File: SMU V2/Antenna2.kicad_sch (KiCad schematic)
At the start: 9 parts, among them J1101 SMA

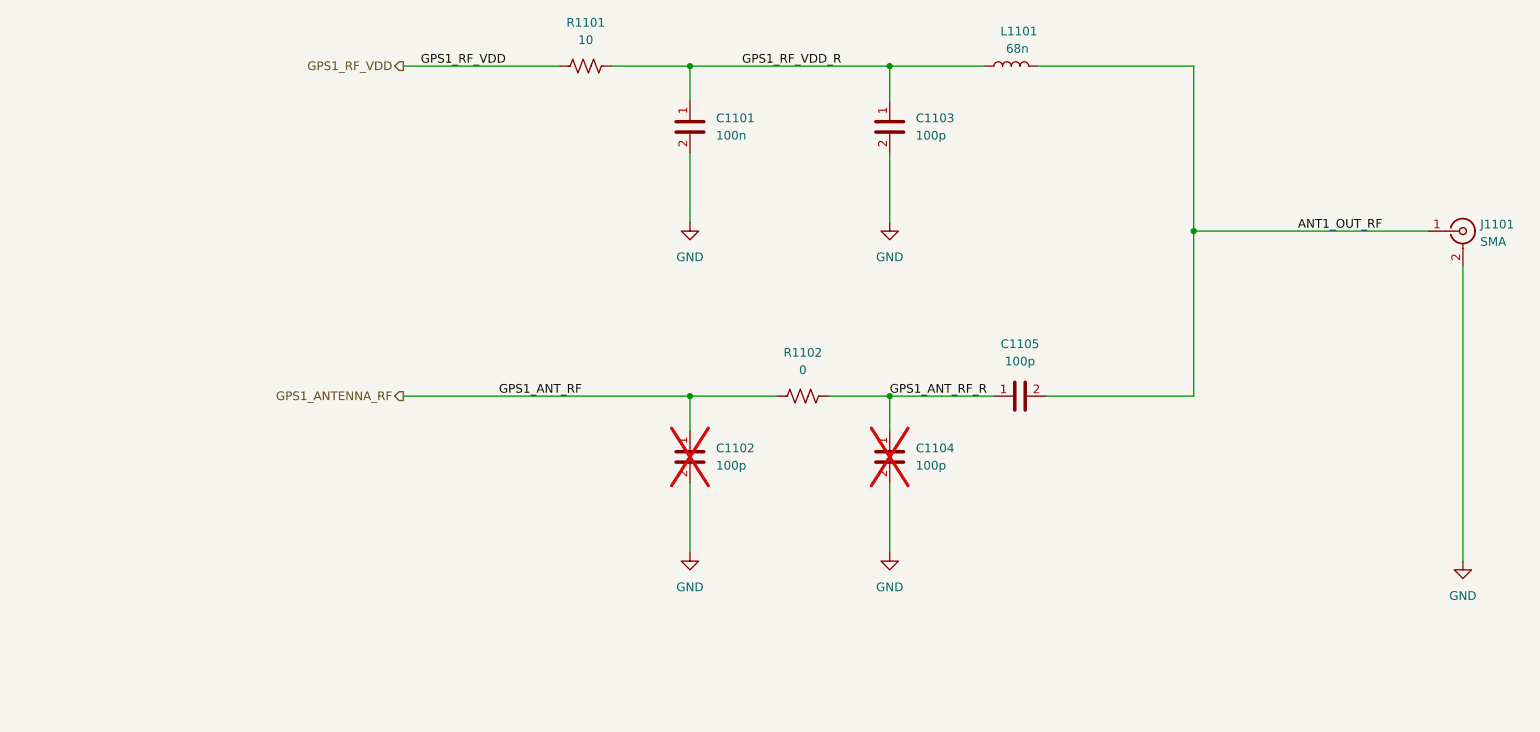
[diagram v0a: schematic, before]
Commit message: v2 layout
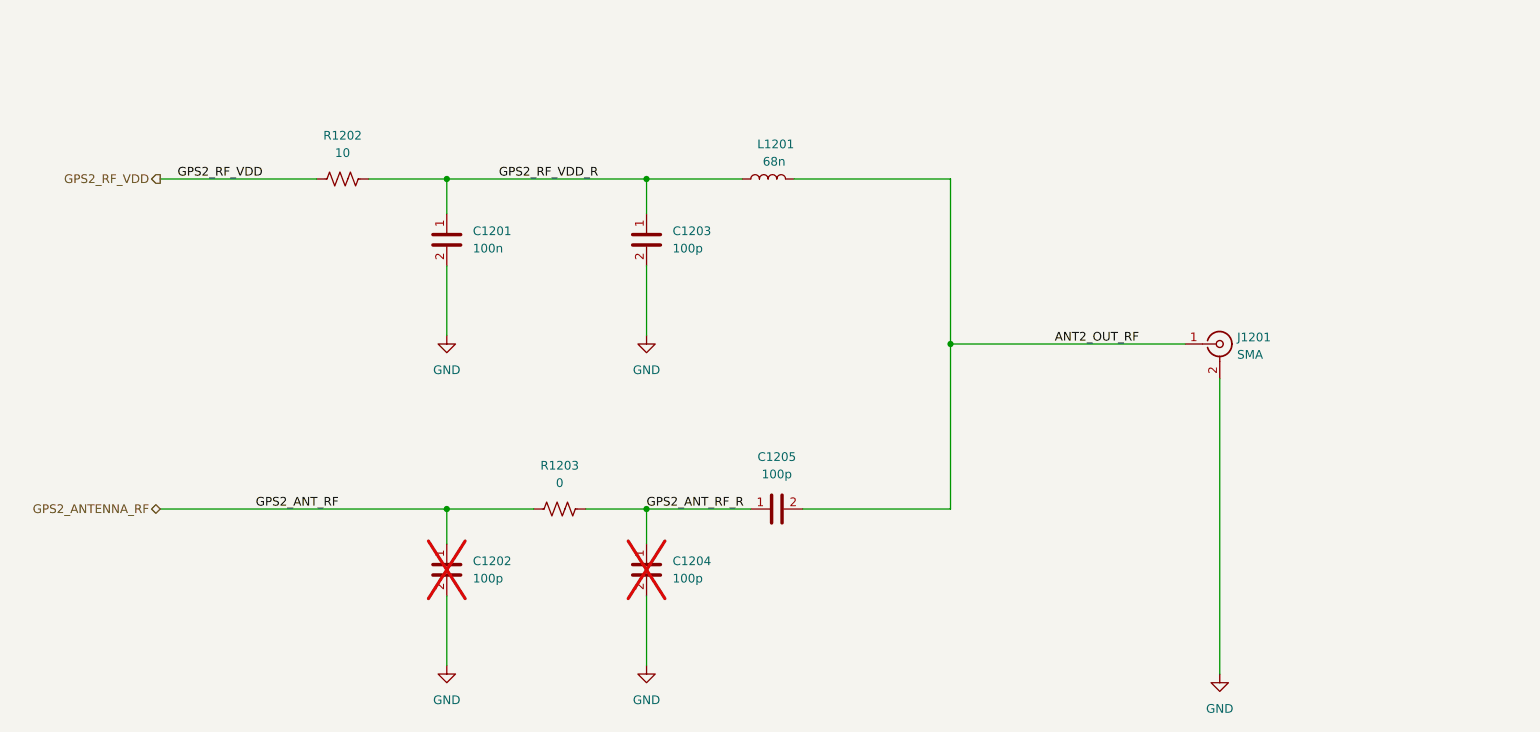
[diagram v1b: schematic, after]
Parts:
- removed C1101: 100n, Capacitor_SMD:C_0402_1005Metric_Pad0.74x0.62mm_HandSolder, symbol bfr_capacitors:CL05B104KB54PNC
- removed C1102, C1103, C1104, C1105: 100p, Capacitor_SMD:C_0402_1005Metric_Pad0.74x0.62mm_HandSolder, symbol bfr_capacitors:0402CG101J500NT
- removed J1101: SMA, bfr_connectors:THT SMA, symbol bfr_connectors:THT_SMA
- removed L1101: 68n, Inductor_SMD:L_0402_1005Metric_Pad0.77x0.64mm_HandSolder, symbol bfr_inductors:LQW15AN68NG0ZD
- removed R1101: 10, Resistor_SMD:R_0402_1005Metric_Pad0.72x0.64mm_HandSolder, symbol bfr_resistors:RMCF0402FT10R0
- removed R1102: 0, Resistor_SMD:R_0402_1005Metric_Pad0.72x0.64mm_HandSolder, symbol bfr_resistors:RMCF0402ZT0R00
- added C1201: 100n, Capacitor_SMD:C_0402_1005Metric_Pad0.74x0.62mm_HandSolder, symbol bfr_capacitors:CL05B104KB54PNC
- added C1202, C1203, C1204, C1205: 100p, Capacitor_SMD:C_0402_1005Metric_Pad0.74x0.62mm_HandSolder, symbol bfr_capacitors:0402CG101J500NT
- added J1201: SMA, bfr_connectors:THT SMA, symbol bfr_connectors:THT_SMA
- added L1201: 68n, Inductor_SMD:L_0402_1005Metric_Pad0.77x0.64mm_HandSolder, symbol bfr_inductors:LQW15AN68NG0ZD
- added R1202: 10, Resistor_SMD:R_0402_1005Metric_Pad0.72x0.64mm_HandSolder, symbol bfr_resistors:RMCF0402FT10R0
- added R1203: 0, Resistor_SMD:R_0402_1005Metric_Pad0.72x0.64mm_HandSolder, symbol bfr_resistors:RMCF0402ZT0R00
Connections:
- net GND: now also C1201.2, C1202.2, C1203.2, C1204.2, J1201.2
- new net ANT2_OUT_RF: C1205.2, J1201.1, L1201.1
- new net GPS2_ANTENNA_RF: C1202.1, R1203.1
- new net GPS2_ANT_RF_R: C1204.1, C1205.1, R1203.2
- new net GPS2_RF_VDD: R1202.1
- new net GPS2_RF_VDD_R: C1201.1, C1203.1, L1201.2, R1202.2
